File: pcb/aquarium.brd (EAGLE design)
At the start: 120.6 x 67 mm, 56 parts, among them J1 PUMP_PWR, J10 DO_IN, J11 LD1117, J12 LEVEL, J13 FLOW, J14 5V, J15 DO, J16 PH, J17 EC_IN, J18 EC, J19 EC_PWR_OUT, J2 EC_OUT, J20 EC_PWR_IN, J21 MCP3424-B, J22 MCP3424-A, J23 GPIO, J24 ADC-3, J25 ADC-4, J26 DS18B20, J27 DS18B20, J28 LD1117, J29 ADC-1, J3 PH_PWR_OUT, J4 PH_PWR_IN, J5 DO_PWR_OUT, J6 DO_PWR_IN, J7 PH_OUT, J8 DO_OUT, J9 PH_IN, Q1 2n3904, Q2 2n3904, Q3 2n3904, Q4 2n3904

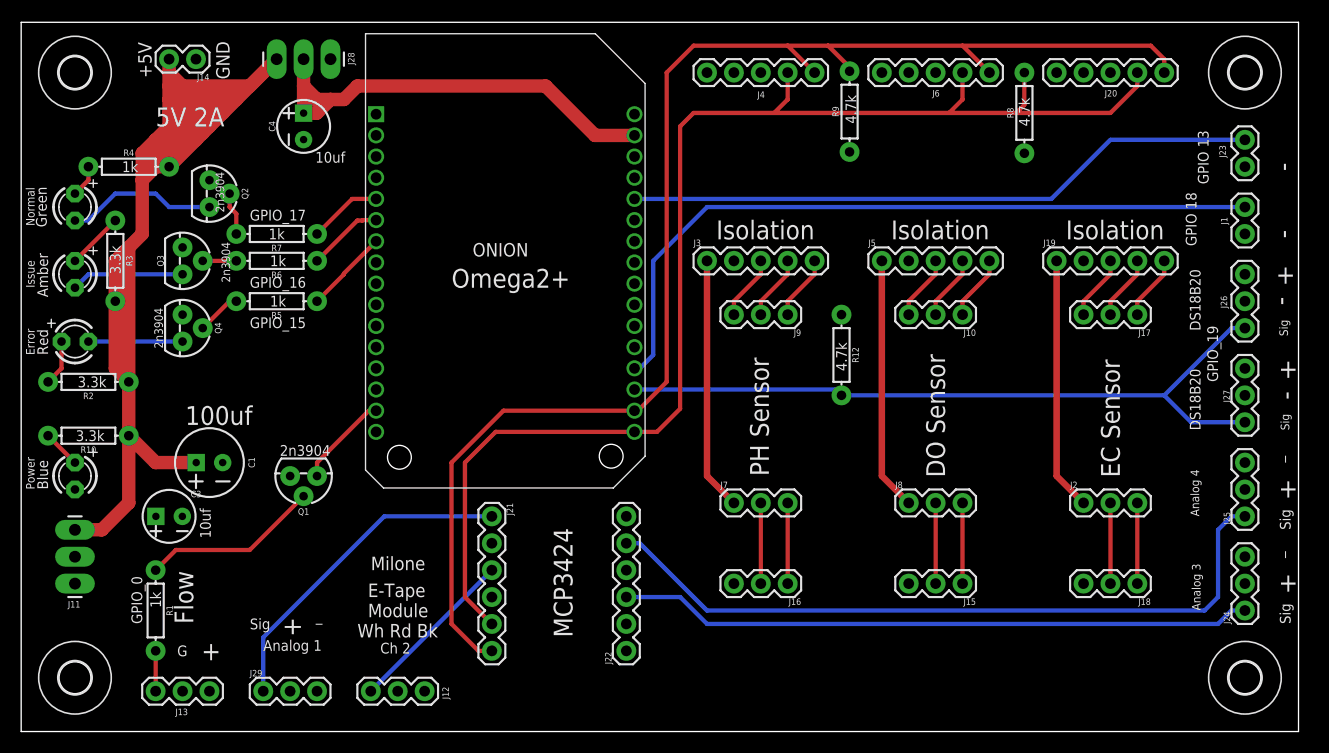
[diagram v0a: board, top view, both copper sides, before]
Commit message: Updating the board to the latest
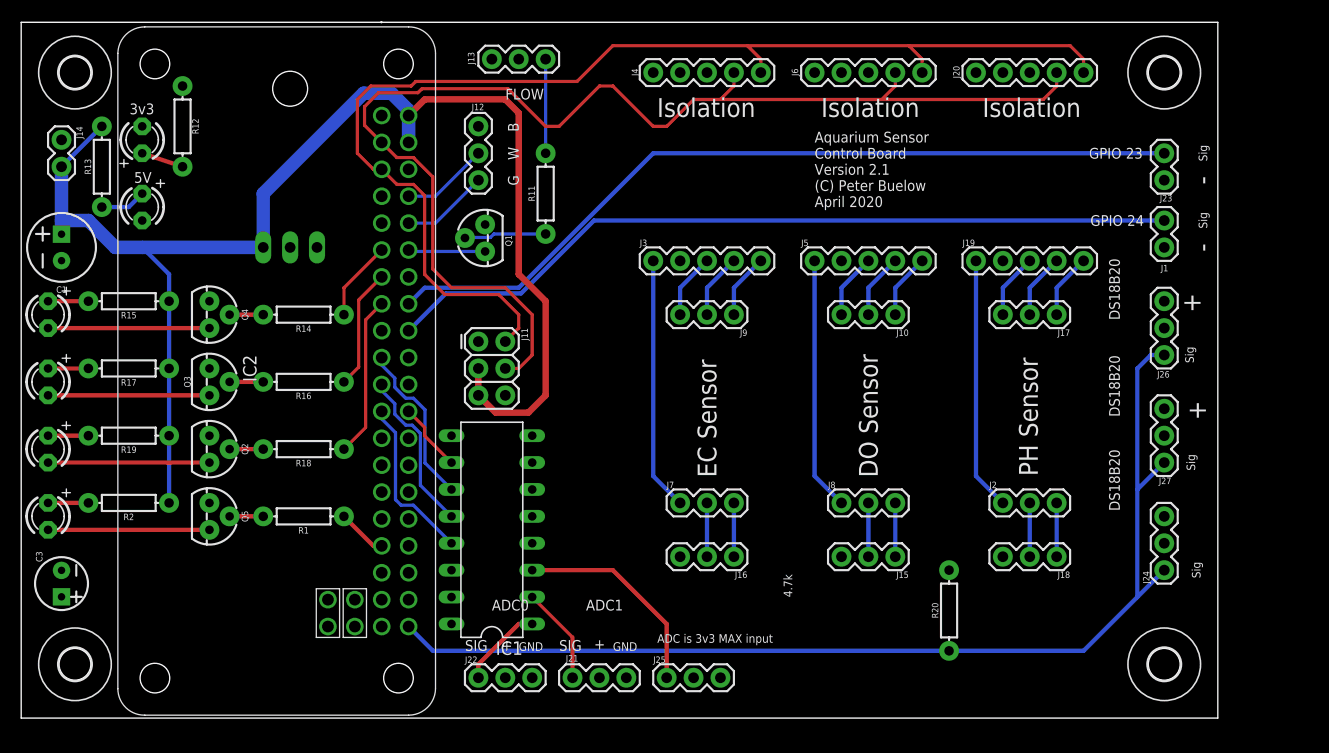
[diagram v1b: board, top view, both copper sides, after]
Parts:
- removed C4: 10uF, SparkFun-Capacitors:CPOL-RADIAL-2.5MM-5MM
- removed J28: LD1117, SparkFun-Connectors:1X03_LONGPADS
- removed J29: ADC-1, SparkFun-Connectors:1X03
- removed ONION: OMEGA2+, OMEGA2_:OMEGA2_PADS
- removed R10: 100, SparkFun-Resistors:AXIAL-0.3
- removed R3: 3.3k, SparkFun-Resistors:AXIAL-0.3
- removed R4, R5, R6, R7: 1k, SparkFun-Resistors:AXIAL-0.3
- removed R8, R9: 4.7k, SparkFun-Resistors:AXIAL-0.3
- added IC1: MCP3008, adafruit:DIL16
- added IC2: PI Zero, Rasbperry_Pi_Zero_W:RASPBERRYPIZEROWV13
- added LDO: LD1117V33, SparkFun-IC-Power:78XXL
- added LED1: 3.3V, adafruit:LED3MM
- added LED2: 2.0V, adafruit:LED3MM
- added Q5: 2n3904, SparkFun-DiscreteSemi:TO-92
- added R11, R13, R14, R15, R16, R17, R18, R19: 1k, SparkFun-Resistors:AXIAL-0.3
- added R20: 4.7k, SparkFun-Resistors:AXIAL-0.3
- J11: value LD1117 -> OLED Display; device SparkFun-Connectors:1X03_LONGPADS -> SparkFun-Connectors:2X3
- J12: value LEVEL -> UART
- J21: value MCP3424-B -> ADC2; device SparkFun-Connectors:1X06 -> SparkFun-Connectors:1X03
- J22: value MCP3424-A -> ADC1; device SparkFun-Connectors:1X06 -> SparkFun-Connectors:1X03
- J24: value ADC-3 -> DS18B20
- J25: value ADC-4 -> ADC3
- R12: value 4.7K -> 100
- R2: value 3.3k -> 1k
- moved R12 65.9 mm to (15.2, 57.1), turned to 90 degrees
- moved J13 65.4 mm to (44.5, 63.5), turned to 0 degrees
- moved J25 56.7 mm to (61.0, 5.08), turned to 0 degrees
- moved J12 54.3 mm to (43.2, 57.1), turned to 270 degrees
- moved J11 44.4 mm to (43.2, 36.8), turned to 270 degrees
- moved Q1 28.3 mm to (43.8, 46.6), turned to 90 degrees
- moved LED4 26.2 mm to (11.4, 49.5)
- moved C1 24.7 mm to (3.81, 45.7), turned to 90 degrees
- moved Q2 24.1 mm to (17.8, 26.7)
- moved LED7 23.0 mm to (2.54, 26.7)
- moved J21 17.0 mm to (52.1, 5.08), turned to 0 degrees
- moved R1 16.6 mm to (26.7, 20.3), turned to 180 degrees
- moved J14 14.8 mm to (3.81, 55.9), turned to 270 degrees
- moved J22 14.2 mm to (43.2, 5.08), turned to 0 degrees
- moved R2 12.0 mm to (10.2, 21.6)
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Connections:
- removed net C1+: J21.1, J29.1
- removed net C2+: J12.1, J21.3
- removed net C3+: J22.3, J24.1
- removed net C4+: J22.5, J25.1
- removed net GPIO_0: ONION.15, Q1.1
- removed net GPIO_13: J23.1, ONION.28
- removed net GPIO_15: ONION.7, R5.P$1
- removed net GPIO_16: ONION.6, R6.P$1
- removed net GPIO_17: ONION.5, R7.P$1
- removed net GPIO_18: J1.1, ONION.20
- removed net GPIO_19: J26.1, J27.1, ONION.19, R12.P$2
- removed net VCC: C4.1, J28.2, ONION.31
- new net 1WIRE: IC2.40, J24.1, J26.1, J27.1, R20.P$1
- new net CH0: IC1.1, J22.1
- new net CH1: IC1.2, J21.1
- new net CH2: IC1.3, J25.1
- new net CLK: IC1.13, IC2.23
- new net CS: IC1.10, IC2.24
- new net GPIO13: IC2.33, R1.P$1
- new net GPIO17: IC2.11, R14.P$1
- new net GPIO18: IC2.12, Q1.1
- new net GPIO22: IC2.15, R18.P$1
- new net GPIO23: IC2.16, J23.1
- new net GPIO24: IC2.18, J1.1
- new net GPIO27: IC2.13, R16.P$1
- new net MISO: IC1.12, IC2.21
- new net MOSI: IC1.11, IC2.19
- new net N$13: Q5.2, R1.P$2
- new net N$14: LED2.A, R2.P$2
- new net N$15: LED2.K, Q5.3
- new net SIG: J13.3, R11.P$2
- new net UART_RX0: IC2.10, J12.3
- new net UART_TX0: IC2.8, J12.2
- net +5V: now also IC2.2, IC2.4, J11.5, LDO.OUT, R13.P$2, R15.P$1, R17.P$1, R19.P$1; no longer J28.3, R10.P$1, R3.P$2, R4.P$2
- net GND: now also IC1.14, IC1.4, IC1.5, IC1.6, IC1.7, IC1.8, IC1.9, IC2.14, IC2.20, IC2.25, IC2.30, IC2.34, IC2.39, IC2.6, IC2.9, J12.1, J21.3, J22.3, J24.2, LDO.IN, LED1.K, Q5.1; no longer C4.2, J12.3, J21.2, J21.4, J22.1, J22.4, J22.6, J24.3, J28.1, J29.3, ONION.1, ONION.32
- net N$1: now also LED1.A, R12.P$1; no longer J13.3, R1.P$2
- net N$11: now also R19.P$2; no longer R4.P$1
- net N$2: now also R11.P$1; no longer R1.P$1
- net N$3: now also R14.P$2; no longer R5.P$2
- net N$4: now also R13.P$1; no longer R10.P$2
- net N$5: now also R16.P$2; no longer R6.P$2
- net N$6: now also R15.P$2; no longer R2.P$2
- net N$7: now also R18.P$2; no longer R7.P$2
- net N$9: now also R17.P$2; no longer R3.P$1
- net SCL: now also IC2.5, J11.2; no longer J21.6, ONION.18, R9.P$2
- net SDA: now also IC2.3, J11.4; no longer J21.5, ONION.17, R8.P$2
- net VDD: now also IC1.15, IC1.16, J21.2, J24.3, LDO.GND, R12.P$2, R20.P$2; no longer J11.2, J12.2, J24.2, J29.2, R12.P$1, R8.P$1, R9.P$1
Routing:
- net 1WIRE: track 0.00 -> 103.7 mm
- net GPIO23: track 0.00 -> 77.2 mm
- net GPIO24: track 0.00 -> 75.7 mm
- net GPIO_19: track 69.2 -> 0.00 mm
- net GPIO_18: track 69.2 -> 0.00 mm
- net C4+: track 68.5 -> 0.00 mm
- net C3+: track 60.0 -> 0.00 mm
- net GPIO_13: track 60.0 -> 0.00 mm
- net VCC: track 43.7 -> 0.00 mm
- net C1+: track 31.4 -> 0.00 mm
- net SCL: track 133.1 -> 112.7 mm
- net CH2: track 0.00 -> 19.9 mm
- net C2+: track 16.2 -> 0.00 mm
- net CLK: track 0.00 -> 15.9 mm
- net MOSI: track 0.00 -> 15.6 mm
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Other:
- board size 120.6 x 67 mm -> 113 x 65.7 mm
- board text added: "3v3"
- board text added: "5V"
- board text added: "ADC is 3v3 MAX input"
- board text added: "ADC0"
- board text added: "ADC1"
- board text added: "Aquarium Sensor Control Board Version 2.1 (C) Peter Buelow April 2020"
- board text added: "B"
- board text added: "FLOW"
- board text added: "GPIO 23"
- board text added: "GPIO 24"
- board text added: "SIG"
- board text added: "W"
- board text removed: "+5V"
- board text removed: "100uf"
- board text removed: "10uf"
- board text removed: "1k"
- board text removed: "2n3904"
- board text removed: "3.3k"
- board text removed: "5V 2A"
- board text removed: "Amber"
- board text removed: "Analog 1"
- board text removed: "Analog 3"
- board text removed: "Analog 4"
- board text removed: "Aquarium Sensor Board Sensor Board (C) Peter Buelow, 2019 Version 1.3"
- board text removed: "Blue"
- board text removed: "Ch 2"
- board text removed: "E-Tape Module Wh Rd Bk"
- board text removed: "Error"
- board text removed: "Flow"
- board text removed: "GPIO 13"
- board text removed: "GPIO 18"
- board text removed: "GPIO_0"
- board text removed: "GPIO_15"
- board text removed: "GPIO_16"
- board text removed: "GPIO_17"
- board text removed: "GPIO_19"
- board text removed: "Green"
- board text removed: "Issue"
- board text removed: "MCP3424"
- board text removed: "Milone"
- board text removed: "Normal"
- board text removed: "Omega2+"
- board text removed: "Power"
- board text removed: "Red"
- board text removed: "_"
